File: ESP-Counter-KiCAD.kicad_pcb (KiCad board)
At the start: 2 copper layers, 110.7 x 107.8 mm, 44 parts, among them J1 Digital_IP, J2 Motor_Ctrl, J3 LED_Indicator, J4 ADC, J5 24V_Input, K2 G2RL-1-DC24, K5 G2RL-1-DC24, U1 ESP_12E_J1, U10 VO615A, U11 AT25xxx-MA, U2 ESP_12E_J2, U3 VO615A, U4 VO615A, U5 VO615A, U6 ULN2801A, U7 VO615A, U8 VO615A, U9 VO615A

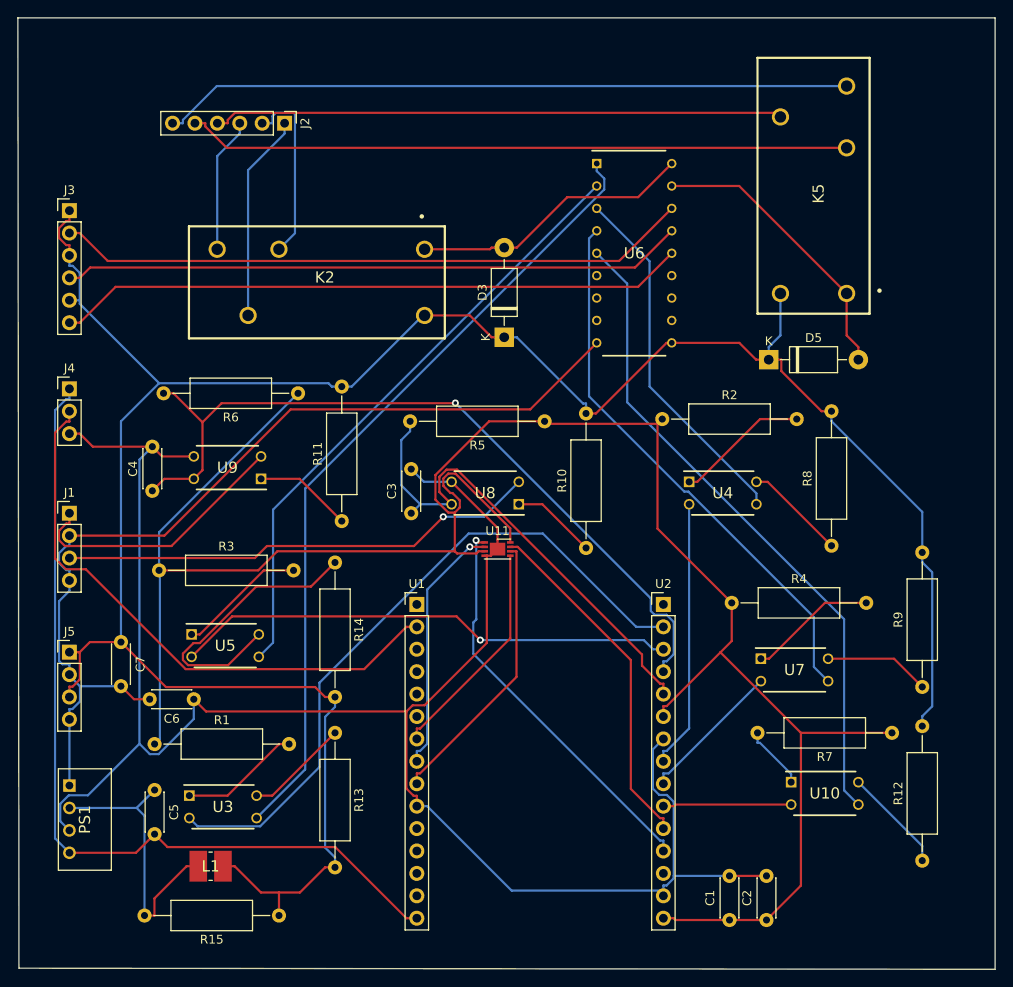
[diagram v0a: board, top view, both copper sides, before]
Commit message: Routing completed - Second iteration
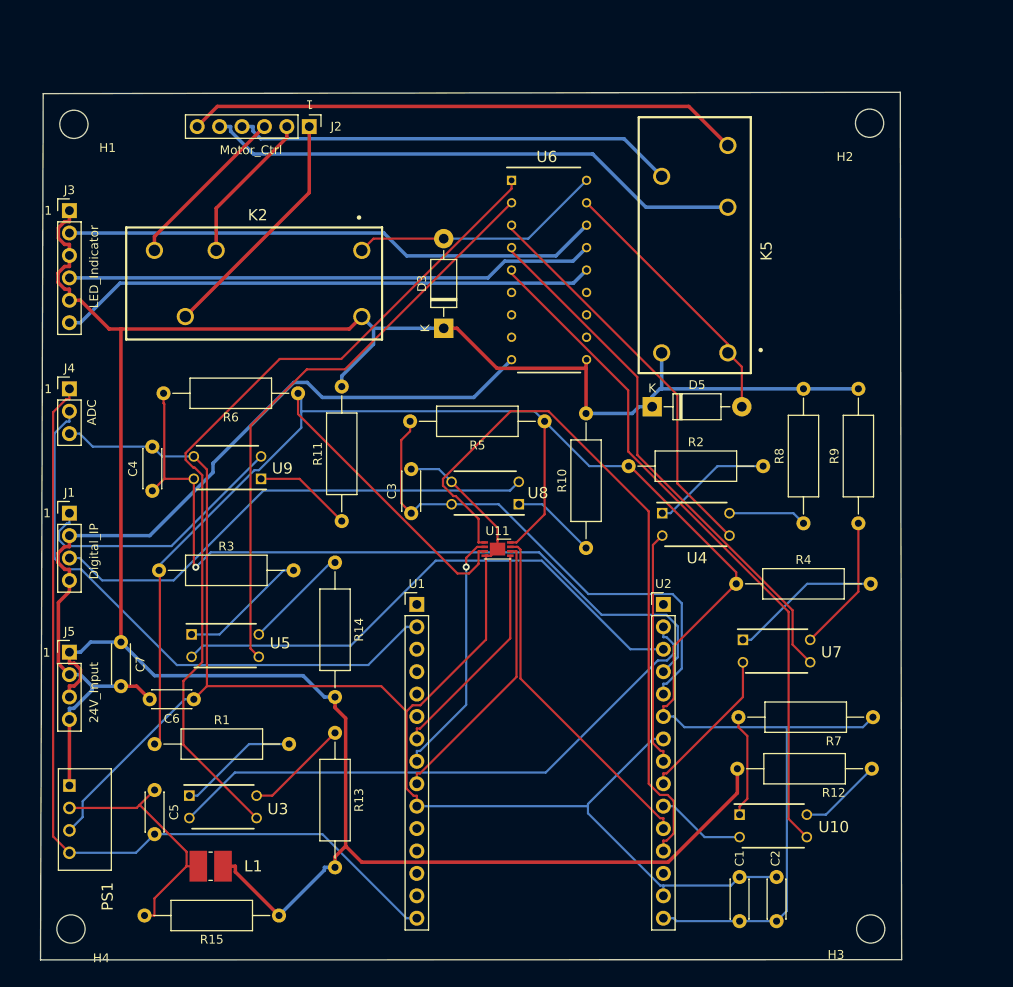
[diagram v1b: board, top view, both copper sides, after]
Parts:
- added H1: ., MountingHole:MountingHole_3.2mm_M3, F.Cu at (88.9, 61.8)
- added H2: ., MountingHole:MountingHole_3.2mm_M3, F.Cu at (179.1, 61.7)
- added H3: ., MountingHole:MountingHole_3.2mm_M3, F.Cu at (179.2, 153.0)
- added H4: ., MountingHole:MountingHole_3.2mm_M3, F.Cu at (88.6, 153.0)
- moved R9 19.9 mm to (177.8, 107.1)
- moved K5 15.1 mm to (165.6, 90.0)
- moved D5 14.2 mm to (154.4, 93.9)
- moved R12 11.9 mm to (179.3, 134.9), turned to 180 degrees
- moved U6 9.84 mm to (142.7, 78.4)
- moved K2 7.11 mm to (123.8, 73.5)
- moved D3 6.93 mm to (130.8, 85.0)
- moved U10 6.91 mm to (168.1, 141.4)
- moved R2 6.55 mm to (151.8, 100.6)
- moved U4 4.68 mm to (159.4, 107.2)
- moved R8 4.07 mm to (171.6, 107.1)
- moved U7 2.95 mm to (168.5, 121.5)
- moved J2 2.82 mm to (115.6, 62.1)
- moved R7 2.80 mm to (179.5, 129.0)
- moved R4 2.22 mm to (164.0, 113.9)
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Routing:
- net CS: track 45.6 -> 81.8 mm, vias 1 -> 0
- net Net-(R14-Pad1): track 32.5 -> 12.0 mm
- net 24V: track 275.7 -> 292.1 mm
- net GND: track 213.1 -> 197.4 mm
- net Stop_NO: track 78.4 -> 62.9 mm
- net Stop_COM: track 64.7 -> 50.2 mm
- net Stop_NC: track 75.2 -> 61.7 mm
- net GPIO5: track 77.8 -> 66.4 mm
- net RED: track 72.0 -> 61.1 mm
- net Orange: track 71.5 -> 61.1 mm
- net Green: track 70.5 -> 60.0 mm
- net GND1: track 109.9 -> 101.7 mm
- net Net-(U3-Pad3): track 90.8 -> 96.8 mm
- net VDD3V3: track 238.0 -> 232.7 mm
- net GPIO4: track 56.9 -> 62.1 mm, vias 1 -> 0
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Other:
- board size 110.7 x 107.8 mm -> 97.6 x 98.3 mm
- net class power added: clearance 0.2, trace_width 0.4, via_dia 0.8, via_drill 0.4
- board text added: "1"
